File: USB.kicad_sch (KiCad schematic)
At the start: 4 parts, among them J1 USB_C_Receptacle_USB2.0_16P, U8 USBLC6-2SC6

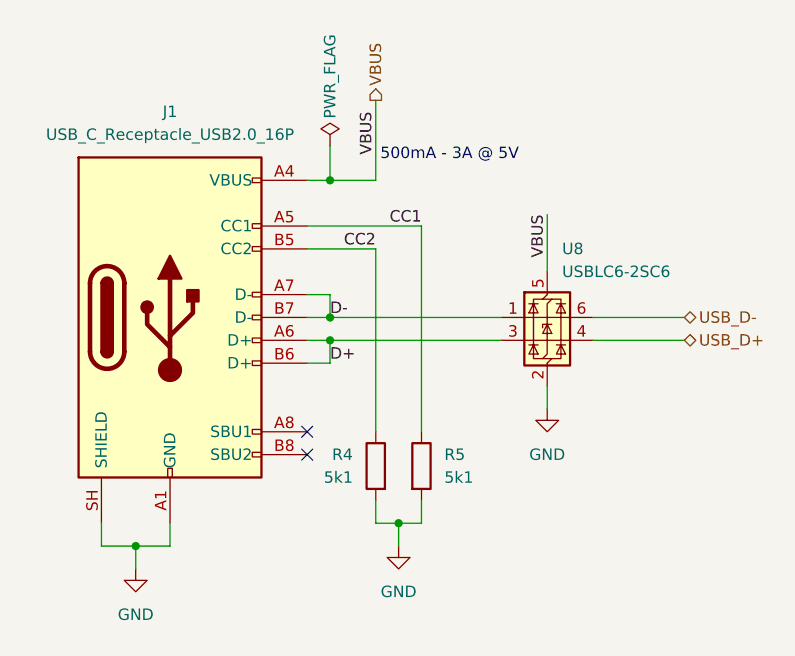
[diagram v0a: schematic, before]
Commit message: more fixes for channels
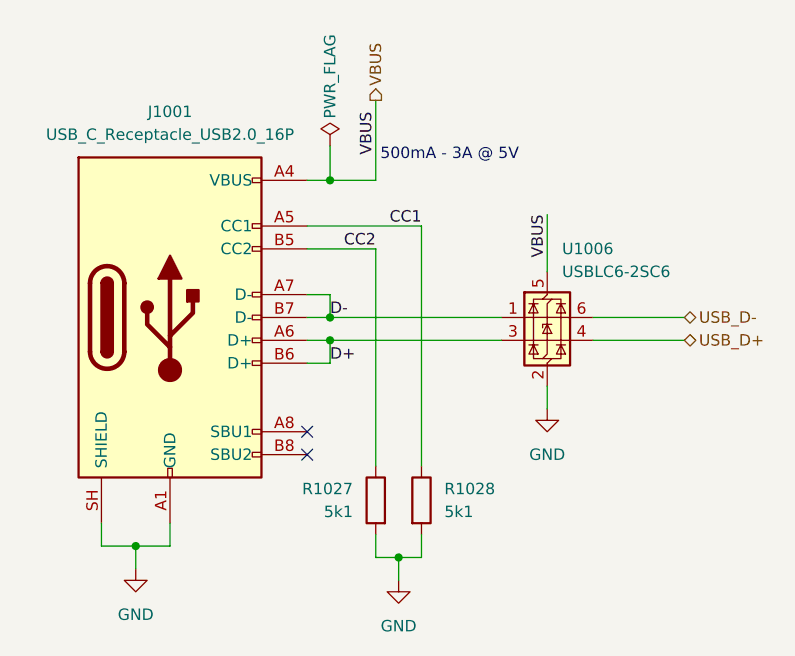
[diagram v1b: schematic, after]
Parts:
- renumbered J1 to J1001, R4 to R1027, R5 to R1028, U8 to U1006
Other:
- moved on the sheet: R1027, R1028
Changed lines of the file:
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@@
 	)
 	(junction
-		(at 147.32 110.49)
+		(at 147.32 114.3)
 		(diameter 0)
 		(color 0 0 0 0)
@@
 	(wire
 		(pts
-			(xy 144.78 110.49) (xy 144.78 107.95)
+			(xy 144.78 114.3) (xy 144.78 111.76)
 		)
 		(stroke
@@
 	(wire
 		(pts
-			(xy 147.32 110.49) (xy 147.32 113.03)
+			(xy 147.32 114.3) (xy 147.32 116.84)
 		)
 		(stroke
@@
 	(wire
 		(pts
-			(xy 149.86 77.47) (xy 149.86 100.33)
+			(xy 149.86 77.47) (xy 149.86 104.14)
 		)
 		(stroke
@@
 	(wire
 		(pts
-			(xy 147.32 110.49) (xy 144.78 110.49)
+			(xy 147.32 114.3) (xy 144.78 114.3)
 		)
 		(stroke
@@
 	(wire
 		(pts
-			(xy 149.86 107.95) (xy 149.86 110.49)
-		)
-		(stroke
-			(width 0)
-			(type default)
-		)
-	)
-	(wire
-		(pts
-			(xy 147.32 110.49) (xy 149.86 110.49)
+			(xy 149.86 111.76) (xy 149.86 114.3)
+		)
+		(stroke
+			(width 0)
+			(type default)
+		)
+	)
+	(wire
+		(pts
+			(xy 147.32 114.3) (xy 149.86 114.3)
 		)
 		(stroke
@@
 	(wire
 		(pts
-			(xy 144.78 100.33) (xy 144.78 80.01)
+			(xy 144.78 104.14) (xy 144.78 80.01)
 		)
 		(stroke
@@
 		(instances
 			(project "VESC6_OPEN_HARDWARE"
-				(path "/8bc2c25a-a1f1-4ce8-b96a-a4f8f4c35079/4c5fe8a6-8c75-4d28-a0d1-00076ab3fe22"
+				(path "/8bc2c25a-a1f1-4ce8-b96a-a4f8f4c35079/1e81ec4a-7813-42c9-8244-ecd5bd9e7dba/a8cef6d1-1c80-4870-a6aa-c1368869a3a7"
 					(reference "#PWR01")
-					(unit 1)
-				)
-			)
-			(project "UBS-C_TYPE-C-31-M-12"
-				(path "/d915b4b4-54fd-4193-8810-936621a064e8"
-					(reference "#PWR07")
 					(unit 1)
 				)
@@
 		(dnp no)
 		(fields_autoplaced yes)
-		(property "Reference" "U8"
+		(property "Reference" "U1006"
 			(at 165.4811 80.01 0)
 			(show_name no)
@@
 		(instances
 			(project "VESC6_OPEN_HARDWARE"
-				(path "/8bc2c25a-a1f1-4ce8-b96a-a4f8f4c35079/4c5fe8a6-8c75-4d28-a0d1-00076ab3fe22"
-					(reference "U8")
-					(unit 1)
-				)
-			)
-			(project "UBS-C_TYPE-C-31-M-12"
-				(path "/d915b4b4-54fd-4193-8810-936621a064e8"
-					(reference "U1")
+				(path "/8bc2c25a-a1f1-4ce8-b96a-a4f8f4c35079/1e81ec4a-7813-42c9-8244-ecd5bd9e7dba/a8cef6d1-1c80-4870-a6aa-c1368869a3a7"
+					(reference "U1006")
 					(unit 1)
 				)
@@
 		(instances
 			(project "VESC6_OPEN_HARDWARE"
-				(path "/8bc2c25a-a1f1-4ce8-b96a-a4f8f4c35079/4c5fe8a6-8c75-4d28-a0d1-00076ab3fe22"
+				(path "/8bc2c25a-a1f1-4ce8-b96a-a4f8f4c35079/1e81ec4a-7813-42c9-8244-ecd5bd9e7dba/a8cef6d1-1c80-4870-a6aa-c1368869a3a7"
 					(reference "#FLG01")
 					(unit 1)
 				)
 			)
-			(project "UBS-C_TYPE-C-31-M-12"
-				(path "/d915b4b4-54fd-4193-8810-936621a064e8"
-					(reference "#FLG01")
-					(unit 1)
-				)
-			)
 		)
 	)
 	(symbol
 		(lib_id "Device:R")
-		(at 149.86 104.14 0)
+		(at 149.86 107.95 0)
 		(unit 1)
 		(body_style 1)
@@
 		(in_pos_files yes)
 		(dnp no)
-		(property "Reference" "R5"
-			(at 152.4 102.8699 0)
+		(property "Reference" "R1028"
+			(at 152.4 106.6799 0)
 			(show_name no)
 			(do_not_autoplace no)
@@
 		)
 		(property "Value" "5k1"
-			(at 152.4 105.4099 0)
+			(at 152.4 109.2199 0)
 			(show_name no)
 			(do_not_autoplace no)
@@
 		)
 		(property "Footprint" "Resistor_SMD:R_0805_2012Metric_Pad1.20x1.40mm_HandSolder"
-			(at 148.082 104.14 90)
+			(at 148.082 107.95 90)
 			(hide yes)
 			(show_name no)
@@
 		)
 		(property "Datasheet" ""
-			(at 149.86 104.14 0)
+			(at 149.86 107.95 0)
 			(hide yes)
 			(show_name no)
@@
 		)
 		(property "Description" "Resistor"
-			(at 149.86 104.14 0)
+			(at 149.86 107.95 0)
 			(hide yes)
 			(show_name no)
@@
 		)
 		(property "LCSC" "C84375"
-			(at 149.86 104.14 0)
+			(at 149.86 107.95 0)
 			(hide yes)
 			(show_name no)
@@
 		(instances
 			(project "VESC6_OPEN_HARDWARE"
-				(path "/8bc2c25a-a1f1-4ce8-b96a-a4f8f4c35079/4c5fe8a6-8c75-4d28-a0d1-00076ab3fe22"
-					(reference "R5")
-					(unit 1)
-				)
-			)
-			(project "UBS-C_TYPE-C-31-M-12"
-				(path "/d915b4b4-54fd-4193-8810-936621a064e8"
-					(reference "R4")
+				(path "/8bc2c25a-a1f1-4ce8-b96a-a4f8f4c35079/1e81ec4a-7813-42c9-8244-ecd5bd9e7dba/a8cef6d1-1c80-4870-a6aa-c1368869a3a7"
+					(reference "R1028")
 					(unit 1)
 				)
@@
 		(dnp no)
 		(fields_autoplaced yes)
-		(property "Reference" "J1"
+		(property "Reference" "J1001"
 			(at 121.92 64.77 0)
 			(show_name no)
@@
 		(instances
 			(project "VESC6_OPEN_HARDWARE"
-				(path "/8bc2c25a-a1f1-4ce8-b96a-a4f8f4c35079/4c5fe8a6-8c75-4d28-a0d1-00076ab3fe22"
-					(reference "J1")
-					(unit 1)
-				)
-			)
-			(project "UBS-C_TYPE-C-31-M-12"
-				(path "/d915b4b4-54fd-4193-8810-936621a064e8"
-					(reference "J1")
+				(path "/8bc2c25a-a1f1-4ce8-b96a-a4f8f4c35079/1e81ec4a-7813-42c9-8244-ecd5bd9e7dba/a8cef6d1-1c80-4870-a6aa-c1368869a3a7"
+					(reference "J1001")
 					(unit 1)
 				)
@@
 	(symbol
 		(lib_id "power:GND")
-		(at 147.32 113.03 0)
+		(at 147.32 116.84 0)
 		(unit 1)
 		(body_style 1)
@@
 		(fields_autoplaced yes)
 		(property "Reference" "#PWR03"
-			(at 147.32 119.38 0)
+			(at 147.32 123.19 0)
 			(hide yes)
 			(show_name no)
@@
 		)
 		(property "Value" "GND"
-			(at 147.32 118.11 0)
+			(at 147.32 121.92 0)
 			(show_name no)
 			(do_not_autoplace no)
@@
 		)
 		(property "Footprint" ""
-			(at 147.32 113.03 0)
+			(at 147.32 116.84 0)
 			(hide yes)
 			(show_name no)
@@
 		)
 		(property "Datasheet" ""
-			(at 147.32 113.03 0)
+			(at 147.32 116.84 0)
 			(hide yes)
 			(show_name no)
@@
 		)
 		(property "Description" "Power symbol creates a global label with name \"GND\" , ground"
-			(at 147.32 113.03 0)
+			(at 147.32 116.84 0)
 			(hide yes)
 			(show_name no)
@@
 		(instances
 			(project "VESC6_OPEN_HARDWARE"
-				(path "/8bc2c25a-a1f1-4ce8-b96a-a4f8f4c35079/4c5fe8a6-8c75-4d28-a0d1-00076ab3fe22"
+				(path "/8bc2c25a-a1f1-4ce8-b96a-a4f8f4c35079/1e81ec4a-7813-42c9-8244-ecd5bd9e7dba/a8cef6d1-1c80-4870-a6aa-c1368869a3a7"
 					(reference "#PWR03")
-					(unit 1)
-				)
-			)
-			(project "UBS-C_TYPE-C-31-M-12"
-				(path "/d915b4b4-54fd-4193-8810-936621a064e8"
-					(reference "#PWR08")
 					(unit 1)
 				)
@@
 		(instances
 			(project "VESC6_OPEN_HARDWARE"
-				(path "/8bc2c25a-a1f1-4ce8-b96a-a4f8f4c35079/4c5fe8a6-8c75-4d28-a0d1-00076ab3fe22"
+				(path "/8bc2c25a-a1f1-4ce8-b96a-a4f8f4c35079/1e81ec4a-7813-42c9-8244-ecd5bd9e7dba/a8cef6d1-1c80-4870-a6aa-c1368869a3a7"
 					(reference "#PWR08")
 					(unit 1)
 				)
 			)
-			(project "UBS-C_TYPE-C-31-M-12"
-				(path "/d915b4b4-54fd-4193-8810-936621a064e8"
-					(reference "#PWR09")
-					(unit 1)
-				)
-			)
 		)
 	)
 	(symbol
 		(lib_id "Device:R")
-		(at 144.78 104.14 0)
+		(at 144.78 107.95 0)
 		(mirror y)
 		(unit 1)
@@
 		(in_pos_files yes)
 		(dnp no)
-		(property "Reference" "R4"
-			(at 142.24 102.8699 0)
+		(property "Reference" "R1027"
+			(at 142.24 106.6799 0)
 			(show_name no)
 			(do_not_autoplace no)
@@
 		)
 		(property "Value" "5k1"
-			(at 142.24 105.4099 0)
+			(at 142.24 109.2199 0)
 			(show_name no)
 			(do_not_autoplace no)
@@
 		)
 		(property "Footprint" "Resistor_SMD:R_0805_2012Metric_Pad1.20x1.40mm_HandSolder"
-			(at 146.558 104.14 90)
+			(at 146.558 107.95 90)
 			(hide yes)
 			(show_name no)
@@
 		)
 		(property "Datasheet" ""
-			(at 144.78 104.14 0)
+			(at 144.78 107.95 0)
 			(hide yes)
 			(show_name no)
@@
 		)
 		(property "Description" "Resistor"
-			(at 144.78 104.14 0)
+			(at 144.78 107.95 0)
 			(hide yes)
 			(show_name no)
@@
 		)
 		(property "LCSC" "C84375"
-			(at 144.78 104.14 0)
+			(at 144.78 107.95 0)
 			(hide yes)
 			(show_name no)
@@
 		(instances
 			(project "VESC6_OPEN_HARDWARE"
-				(path "/8bc2c25a-a1f1-4ce8-b96a-a4f8f4c35079/4c5fe8a6-8c75-4d28-a0d1-00076ab3fe22"
-					(reference "R4")
+				(path "/8bc2c25a-a1f1-4ce8-b96a-a4f8f4c35079/1e81ec4a-7813-42c9-8244-ecd5bd9e7dba/a8cef6d1-1c80-4870-a6aa-c1368869a3a7"
+					(reference "R1027")
 					(unit 1)
 				)
-			)
-			(project "UBS-C_TYPE-C-31-M-12"
-				(path "/d915b4b4-54fd-4193-8810-936621a064e8"
-					(reference "R5")
-					(unit 1)
-				)
